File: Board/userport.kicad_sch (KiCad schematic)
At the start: 11 parts, among them P1 PETUSERPORT, U16 LSF0204Q, U17 LSF0204Q, U18 LSF0204Q, U19 LSF0204Q, U23 74LVC1G00

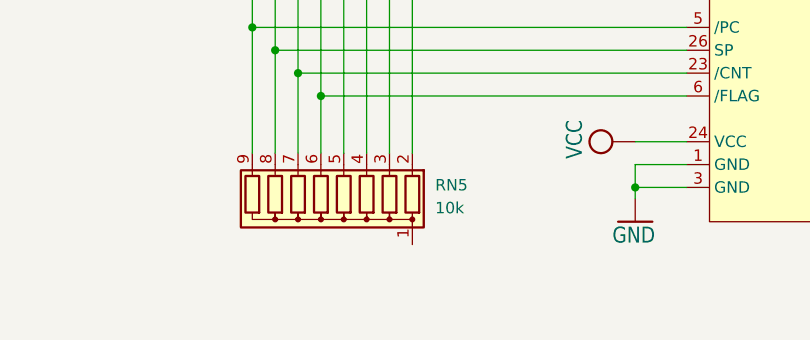
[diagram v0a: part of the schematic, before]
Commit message: full connect, starting on prod
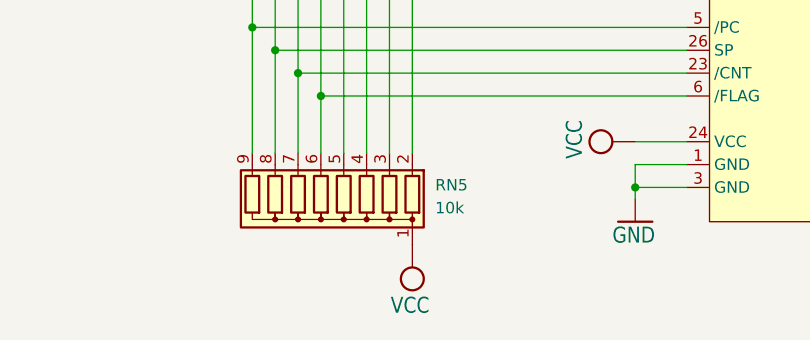
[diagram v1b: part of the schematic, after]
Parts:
- P1: footprint csa_petio_v1:FLAT24 -> csa_petio_v1:FLAT24_IDC
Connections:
- net VCC: now also RN5.1 (common)
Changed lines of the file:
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@@
+	)
+	(symbol
+		(lib_id "csa_petio_v1-eagle-import:VCC")
+		(at 125.73 186.69 180)
+		(unit 1)
+		(exclude_from_sim no)
+		(in_bom yes)
+		(on_board yes)
+		(dnp no)
+		(property "Reference" "#V021"
+			(at 125.73 186.69 0)
+			(effects
+				(font
+					(size 1.27 1.27)
+				)
+				(hide yes)
+			)
+		)
+		(property "Value" "VCC"
+			(at 127.635 189.865 0)
+			(effects
+				(font
+					(size 1.778 1.5113)
+				)
+				(justify left bottom)
+			)
+		)
+		(property "Footprint" ""
+			(at 125.73 186.69 0)
+			(effects
+				(font
+					(size 1.27 1.27)
+				)
+				(hide yes)
+			)
+		)
+		(property "Datasheet" ""
+			(at 125.73 186.69 0)
+			(effects
+				(font
+					(size 1.27 1.27)
+				)
+				(hide yes)
+			)
+		)
+		(property "Description" ""
+			(at 125.73 186.69 0)
+			(effects
+				(font
+					(size 1.27 1.27)
+				)
+				(hide yes)
+			)
+		)
+		(pin "1"
+		)
+		(instances
+			(project "csa_petio_v1"
+				(path "/e52c695d-6540-4a56-9880-06c7d9f215a5/7c8914b4-a2ef-4231-b3f7-1105ec77241e"
+					(reference "#V021")
+					(unit 1)
+				)
+			)
+		)
 	)
 	(symbol
@@
 			)
 		)
-		(property "Footprint" "csa_petio_v1:FLAT24"
+		(property "Footprint" "csa_petio_v1:FLAT24_IDC"
 			(at 176.53 60.96 0)
 			(effects
